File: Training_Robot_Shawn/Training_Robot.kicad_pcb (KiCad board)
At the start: 4 copper layers, 87.5 x 91.5 mm, 26 parts, among them J1 Conn_01x04_Pin, J2 Conn_01x04_Pin, J3 Conn_01x04_Pin, J6 Conn_01x08_Socket, M1 FrontL, M2 FrontR, M3 BackL, M4 BackR, SW1 SW_SPDT_312, U3 ESP32-S3-DevKitC

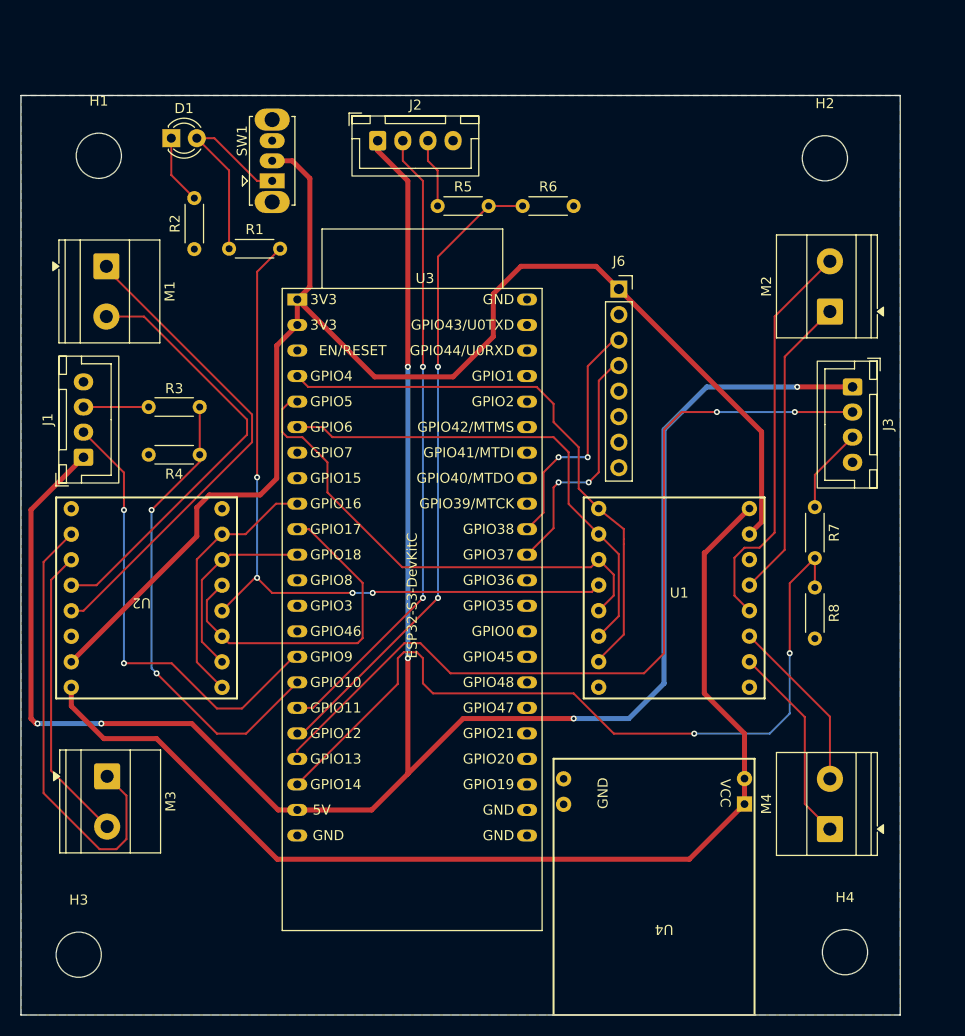
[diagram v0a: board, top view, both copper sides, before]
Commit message: add uncompleted layout
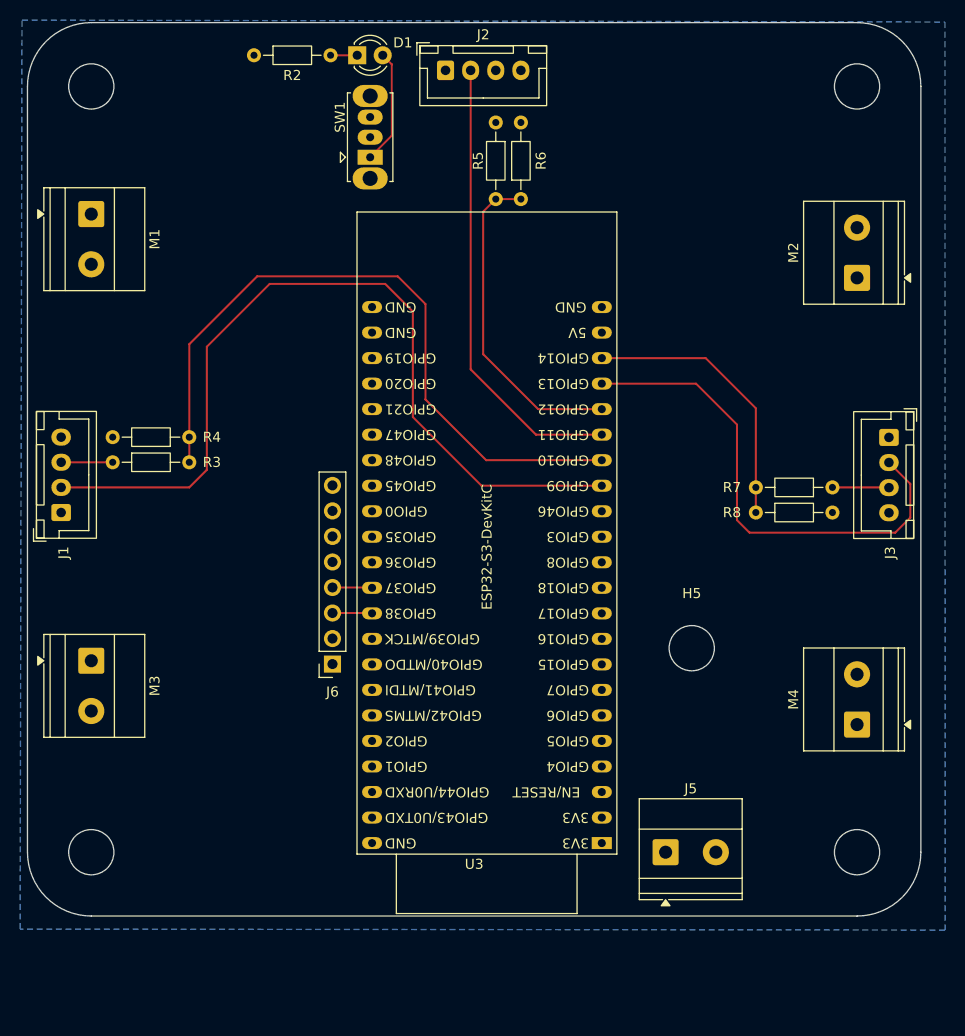
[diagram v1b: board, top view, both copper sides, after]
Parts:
- removed R1: 10K, Resistor_THT:R_Axial_DIN0204_L3.6mm_D1.6mm_P5.08mm_Horizontal
- removed U1, U2: ~, MARS Custom Footprints:TB6612FNG Breakout
- removed U4: ~, MARS Custom Footprints:USB PD Module
- added H5: MountingHole, MountingHole:MountingHole_4.5mm, F.Cu at (123.2, 94.0)
- added J5: Conn_01x02_Pin, TerminalBlock_Phoenix:TerminalBlock_Phoenix_MKDS-1,5-2_1x02_P5.00mm_Horizontal, F.Cu at (120.7, 114.3)
- R2: value 10K -> 180; footprint Resistor_THT:R_Axial_DIN0204_L3.6mm_D1.6mm_P5.08mm_Horizontal -> Resistor_THT:R_Axial_DIN0204_L3.6mm_D1.6mm_P7.62mm_Horizontal
- R3, R4, R5, R6, R7, R8: footprint Resistor_THT:R_Axial_DIN0204_L3.6mm_D1.6mm_P5.08mm_Horizontal -> Resistor_THT:R_Axial_DIN0204_L3.6mm_D1.6mm_P7.62mm_Horizontal
- U3: footprint PCM_Espressif:ESP32-S3-DevKitC -> Espressif:ESP32-S3-DevKitC
- moved U3 62.0 mm to (114.3, 113.4), turned to 180 degrees
- moved J6 47.0 mm to (87.5, 95.6), turned to 180 degrees
- moved D1 20.3 mm to (90.0, 35.0)
- moved R2 20.2 mm to (79.7, 35.0), turned to 0 degrees
- moved M3 11.6 mm to (63.5, 95.2)
- moved M4 10.7 mm to (139.7, 101.6)
- moved H3 10.3 mm to (63.5, 114.3)
- moved R5 10.1 mm to (103.8, 41.7), turned to -90 degrees
- moved SW1 10.0 mm to (91.2, 45.1)
- moved H4 10.0 mm to (139.7, 114.3)
- moved J2 9.72 mm to (98.8, 36.5)
- moved R8 9.49 mm to (129.6, 80.5), turned to 0 degrees
- moved H2 7.83 mm to (139.7, 38.1)
- moved H1 6.94 mm to (63.5, 38.1)
- moved R3 6.56 mm to (65.6, 75.5)
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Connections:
- D1 pad 2: Net-(D1-A) -> /STBY
- SW1 pad 1: Net-(D1-A) -> /STBY
- U3 pad 21: +5V -> unconnected-(U3-5V-Pad21)
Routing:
- net +5V: track 210.2 -> 0.00 mm, vias 6 -> 0
- net +12V: track 110.4 -> 0.00 mm
- net /STBY: track 73.5 -> 11.4 mm, vias 4 -> 0
- net /R_US_ECHO: track 81.0 -> 27.8 mm, vias 2 -> 0
- net /RIGHT_FORWARD: track 49.5 -> 0.00 mm
- net /RIGHT_BACKWARD: track 49.2 -> 0.00 mm
- net /FL+: track 48.4 -> 0.00 mm
- net /BL+: track 44.9 -> 0.00 mm
- net /FL-: track 43.4 -> 0.00 mm
- net /FR-: track 40.2 -> 0.00 mm
- net /RIGHT_EN: track 39.0 -> 0.00 mm
- net /L_US_TRIG: track 45.9 -> 83.8 mm, vias 2 -> 0
- net /R_US_TRIG: track 85.6 -> 49.4 mm, vias 2 -> 0
- net /LEFT_FORWARD: track 35.0 -> 0.00 mm
- net /F_US_ECHO: track 64.1 -> 32.5 mm, vias 2 -> 0
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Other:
- board size 87.5 x 91.5 mm -> 88.9 x 88.9 mm
